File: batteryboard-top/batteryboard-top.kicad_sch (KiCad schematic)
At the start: 6 parts, among them J1 FLE-105-01-G-DV-A, J2 FLE-105-01-G-DV-A

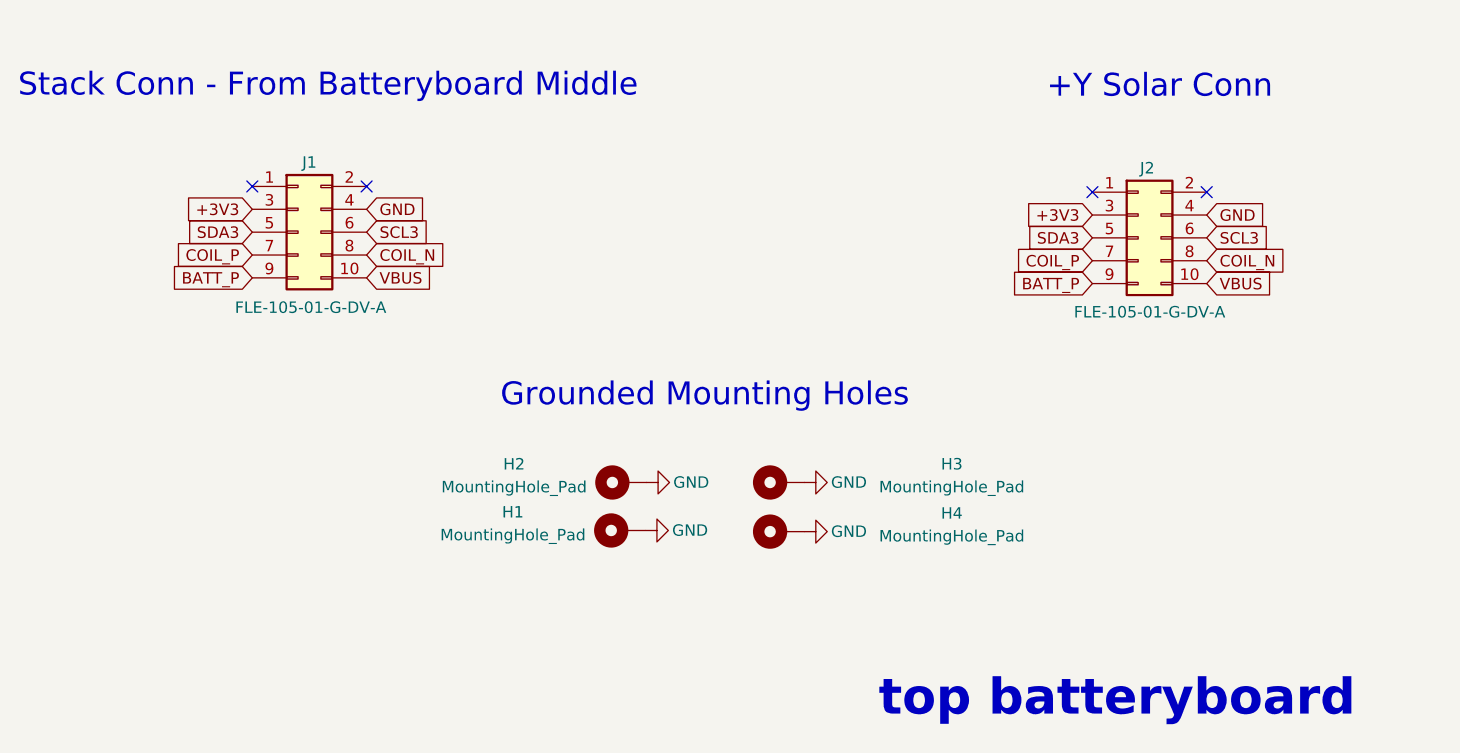
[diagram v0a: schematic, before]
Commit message: Some changes
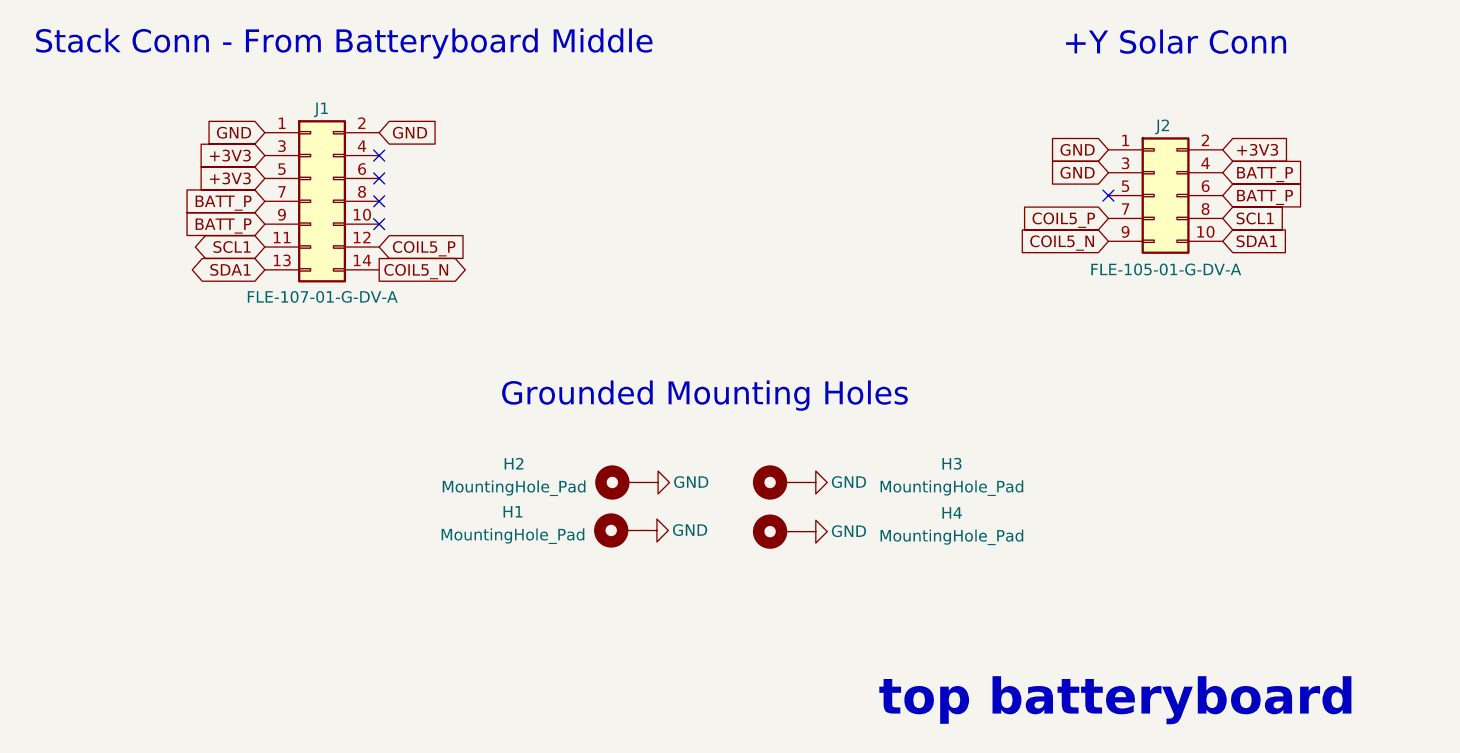
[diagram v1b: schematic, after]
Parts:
- removed J1: FLE-105-01-G-DV-A, batteryboard:SAMTEC_FLE-105-01-G-DV-A, symbol Connector_Generic:Conn_02x05_Odd_Even
- added J1: FLE-107-01-G-DV-A, batteryboard:SAMTEC_FLE-107-01-G-DV-A, symbol Connector_Generic:Conn_02x07_Odd_Even
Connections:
- net SCL3 is gone; now on net BATT_P: J2.6 (Pin_6)
- net +3V3: now also J2.2 (Pin_2), J1.3 (Pin_3), J1.5 (Pin_5); no longer J2.3 (Pin_3)
- net BATT_P: now also J2.4 (Pin_4), J1.7 (Pin_7), J1.9 (Pin_9); no longer J2.9 (Pin_9)
- net GND: now also J2.1 (Pin_1), J2.3 (Pin_3), J1.1 (Pin_1), J1.2 (Pin_2); no longer J2.4 (Pin_4)
- net COIL_N renamed SCL1
- net SCL1: now also J1.11 (Pin_11)
- net COIL_P renamed COIL5_P
- net COIL5_P: now also J1.12 (Pin_12)
- net SDA3: no longer names the net of J2.5 (Pin_5)
- net VBUS renamed SDA1
- net SDA1: now also J1.13 (Pin_13)
- new net COIL5_N: J1.14 (Pin_14), J2.9 (Pin_9)
- no-connect marks 4 -> 5
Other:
- moved on the sheet: J2
